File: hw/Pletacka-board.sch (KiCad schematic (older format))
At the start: 5 parts, among them J4 Conn_01x02_Female, J5 Conn_01x03_Female

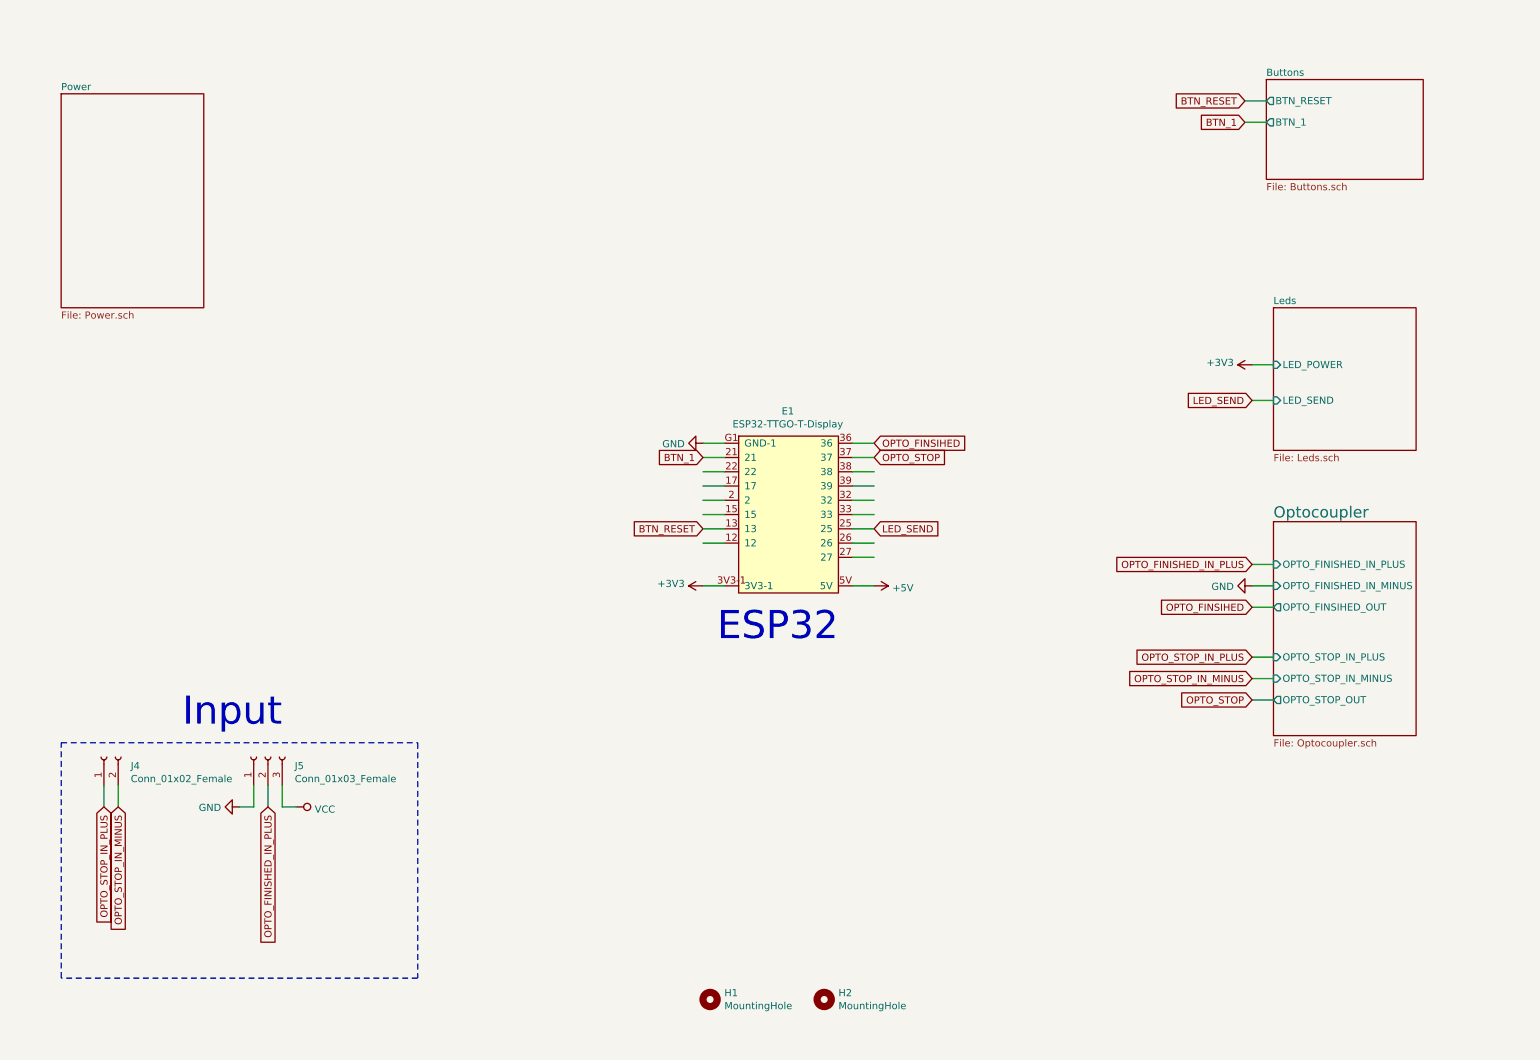
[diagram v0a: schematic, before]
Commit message: Update improve schema and broke board
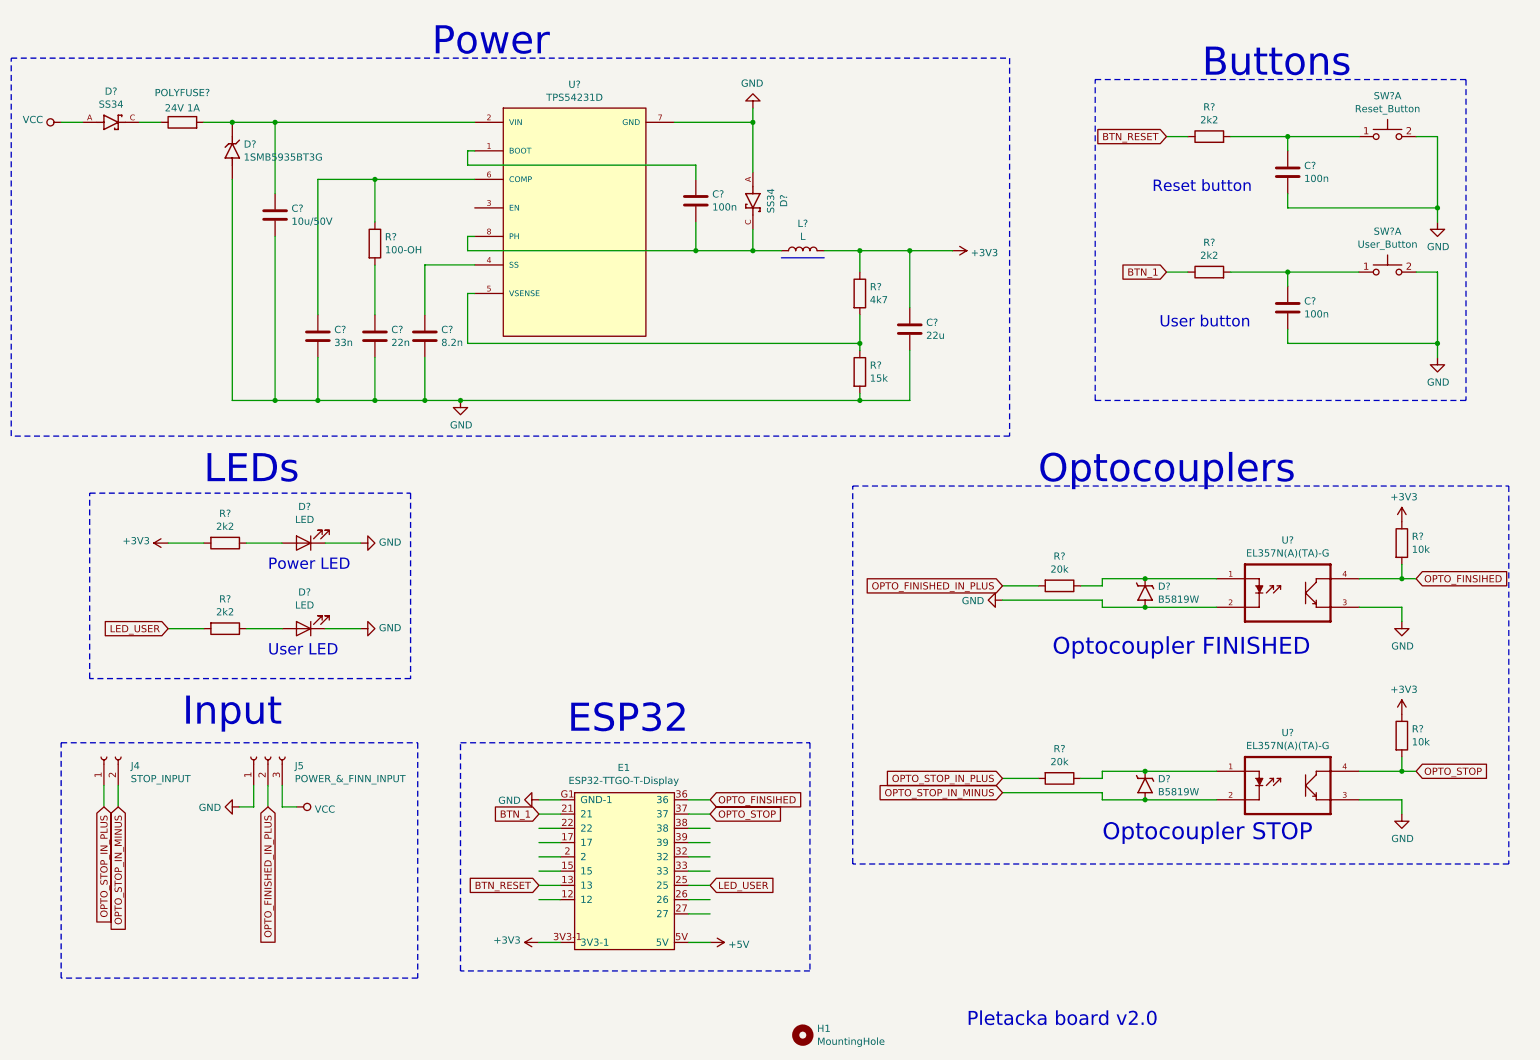
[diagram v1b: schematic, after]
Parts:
- removed H2: MountingHole, MountingHole:MountingHole_2.7mm_M2.5_Pad, symbol Mechanical:MountingHole
- added C? (x3): 100n, Capacitor_SMD:C_0603_1608Metric, symbol Device:C
- added C?: 10u/50V, Capacitor_SMD:C_1206_3216Metric, symbol Device:C
- added C?: 8.2n, Capacitor_SMD:C_0603_1608Metric, symbol Device:C
- added C?: 22n, Capacitor_SMD:C_0603_1608Metric, symbol Device:C
- added C?: 33n, Capacitor_SMD:C_0603_1608Metric, symbol Device:C
- added C?: 22u, Capacitor_SMD:C_0603_1608Metric, symbol Device:C
- added D? (x2): LED, LED_SMD:LED_0603_1608Metric, symbol Device:LED
- added D? (x2): B5819W, B5819W:B5819W_SOD-123, symbol B5819W:B5819W
- added D?: 1SMB5935BT3G, 1SMB5935BT3G:DIOM5436X247N, symbol 1SMB5935BT3G:1SMB5935BT3G
- added D? (x2): SS34, SS34:SMA, symbol SS34:SS34
- added L?: L, Inductor_SMD:L_TDK_SLF7045, symbol Device:L
- added POLYFUSE?: 24V 1A, Resistor_SMD:R_1206_3216Metric, symbol Device:R
- added R? (x4): 2k2, Resistor_SMD:R_0603_1608Metric, symbol Device:R
- added R? (x2): 20k, Resistor_SMD:R_0603_1608Metric, symbol Device:R
- added R? (x2): 10k, Resistor_SMD:R_0603_1608Metric, symbol Device:R
- added R?: 100-OH, Resistor_SMD:R_0603_1608Metric, symbol Device:R
- added R?: 4k7, Resistor_SMD:R_0603_1608Metric, symbol Device:R
- added R?: 15k, Resistor_SMD:R_0603_1608Metric, symbol Device:R
- added SW?: Reset_Button, Button_SMD:SW_SPST_SKQG_WithStem, symbol Switch:SW_Push_Dual_x2
- added SW?: User_Button, Button_SMD:SW_SPST_SKQG_WithStem, symbol Switch:SW_Push_Dual_x2
- added U? (x2): EL357N(A)(TA)-G, EL357N_A__TA_-G:SOP254P700X200-4N, symbol EL357N_A__TA_-G:EL357N(A)(TA)-G
- added U?: TPS54231D, SOIC127P599X175-8N, symbol TPS54231D:TPS54231D
- J4: value Conn_01x02_Female -> STOP_INPUT
- J5: value Conn_01x03_Female -> POWER_&_FINN_INPUT
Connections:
- net labels added: LED_USER
- net labels removed: LED_SEND
- wire segments 36 -> 129
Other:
- note added: "Buttons"
- note added: "LEDs"
- note added: "Optocoupler FINISHED"
- note added: "Optocoupler STOP"
- note added: "Optocouplers"
- note added: "Pletacka board v2.0"
- note added: "Power"
- note added: "Power LED"
- note added: "Reset button"
- note added: "User LED"
- note added: "User button"
- moved on the sheet: E1, H1
